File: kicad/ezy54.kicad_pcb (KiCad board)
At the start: 2 copper layers, 141.5 x 124.7 mm, 63 parts

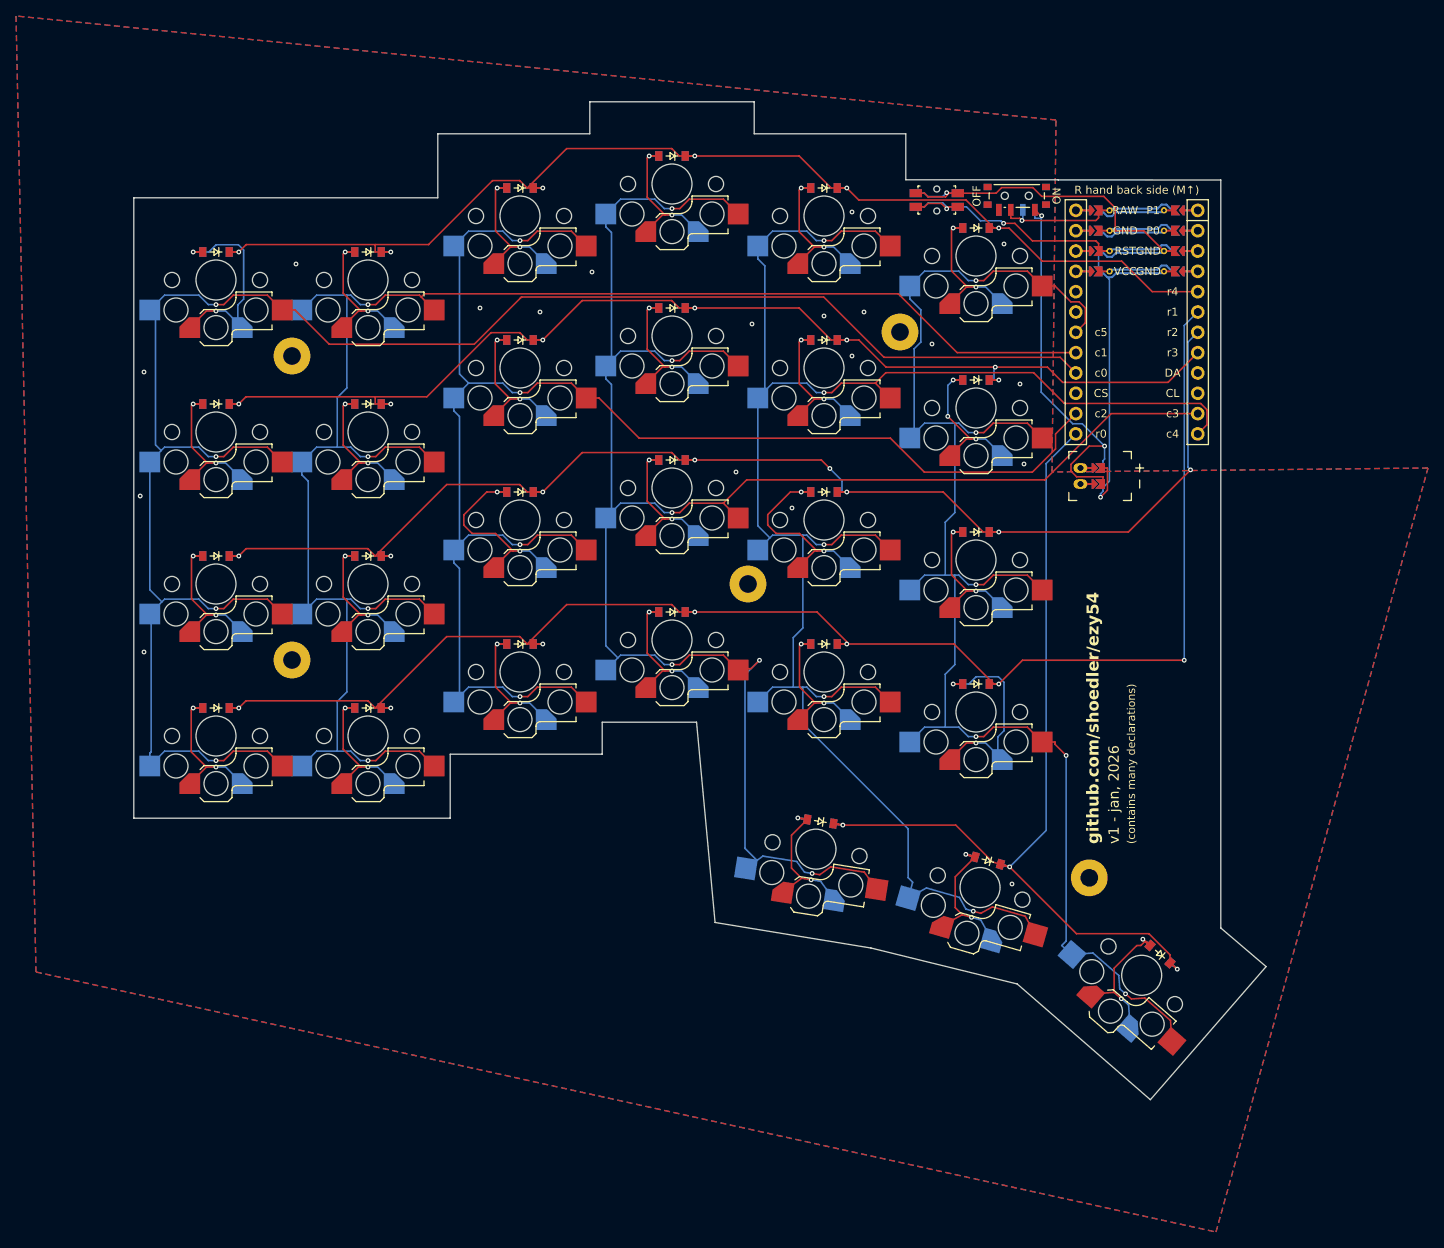
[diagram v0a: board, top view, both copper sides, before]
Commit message: Adds pcb rev1 files
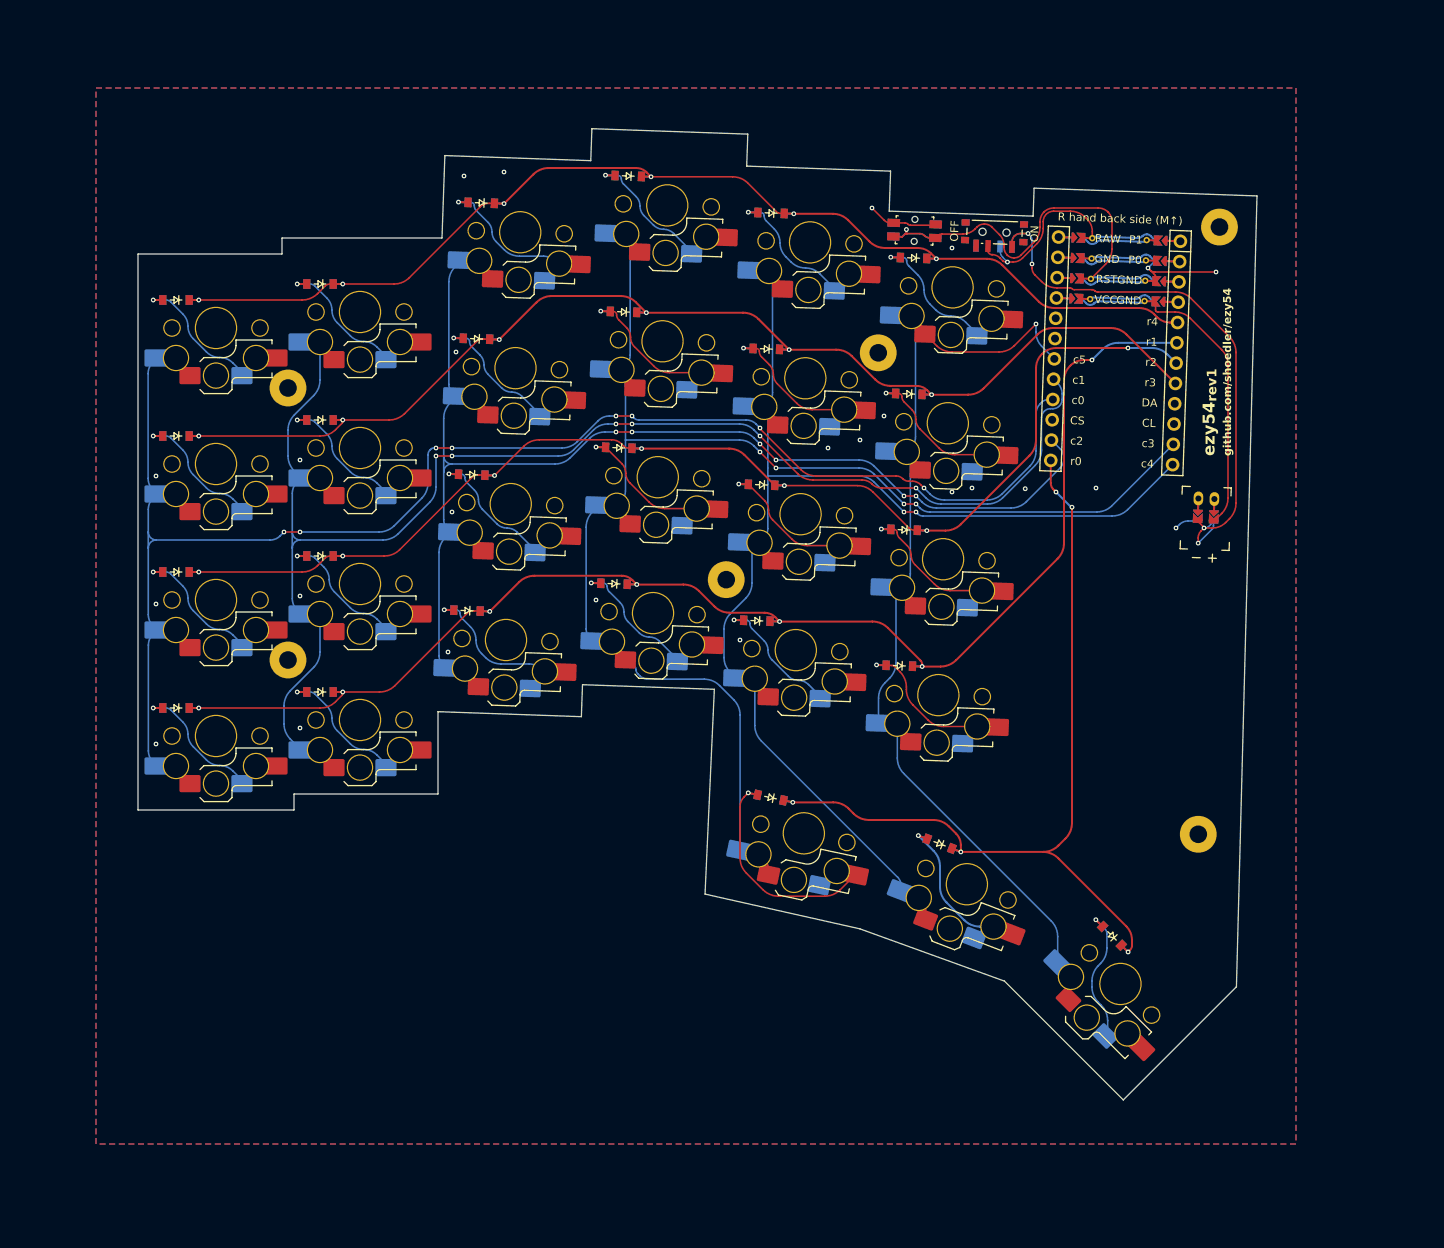
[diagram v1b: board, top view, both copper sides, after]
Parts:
- added MH6: , ceoloide:mounting_hole_npth, F.Cu at (275.4, 86.4)
- moved MH5 64.4 mm to (272.8, 162.3), turned to -2 degrees
- moved MH4 58.7 mm to (213.8, 130.5), turned to -2 degrees
- moved JST1 16.0 mm to (273.8, 120.3), turned to -2 degrees
- moved D21 9.85 mm to (235.4, 141.2), turned to 178 degrees
- moved D22 8.99 mm to (236.0, 124.2), turned to 178 degrees
- moved D17 8.89 mm to (217.6, 135.6), turned to 178 degrees
- moved D24 8.66 mm to (237.2, 90.2), turned to 178 degrees
- moved D23 8.57 mm to (236.6, 107.2), turned to 178 degrees
- moved D13 8.06 mm to (199.8, 131.0), turned to 178 degrees
- moved D18 7.85 mm to (218.2, 118.6), turned to 178 degrees
- moved D9 7.83 mm to (181.4, 134.3), turned to 178 degrees
- moved D4 7.81 mm to (145.0, 95.5)
- moved D20 7.32 mm to (219.4, 84.6), turned to 178 degrees
- moved D19 7.30 mm to (218.8, 101.6), turned to 178 degrees
- moved D8 7.21 mm to (163.0, 93.5)
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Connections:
- S1 pad : (no net) -> GND
- S10 pad : (no net) -> GND
- S11 pad : (no net) -> GND
- S12 pad : (no net) -> GND
- S13 pad : (no net) -> GND
- S14 pad : (no net) -> GND
- S15 pad : (no net) -> GND
- S16 pad : (no net) -> GND
- S17 pad : (no net) -> GND
- S18 pad : (no net) -> GND
- S19 pad : (no net) -> GND
- S2 pad : (no net) -> GND
- S20 pad : (no net) -> GND
- S21 pad : (no net) -> GND
- S22 pad : (no net) -> GND
- S23 pad : (no net) -> GND
- S24 pad : (no net) -> GND
- S25 pad : (no net) -> GND
- S26 pad : (no net) -> GND
- S27 pad : (no net) -> GND
- S3 pad : (no net) -> GND
- S4 pad : (no net) -> GND
- S5 pad : (no net) -> GND
- S6 pad : (no net) -> GND
- S7 pad : (no net) -> GND
- S8 pad : (no net) -> GND
- S9 pad : (no net) -> GND
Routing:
- net c4: track 232.4 -> 169.8 mm, vias 5 -> 2
- net c5: track 193.3 -> 139.5 mm, vias 6 -> 1
- net c3: track 244.2 -> 192.9 mm, vias 6 -> 4
- net c2: track 200.9 -> 165.0 mm, vias 4 -> 6
- net c0: track 239.8 -> 210.5 mm, vias 4 -> 8
- net BAT_P: track 49.8 -> 74.4 mm, vias 2 -> 4
- net GND: track 109.5 -> 86.7 mm, vias 21 -> 25
- net RST: track 42.3 -> 59.9 mm, vias 2 -> 1
- net c1: track 218.8 -> 203.4 mm, vias 4 -> 6
- net c3_r0: track 20.0 -> 33.9 mm, vias 2 -> 1
- net r1: track 188.9 -> 175.8 mm
- net RAW: track 24.7 -> 32.1 mm
- net r3: track 145.9 -> 152.7 mm, vias 7 -> 6
- net r2: track 162.8 -> 157.3 mm, vias 8 -> 7
- net c2_r1: track 19.0 -> 23.3 mm, vias 2 -> 1
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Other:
- board size 141.5 x 124.7 mm -> 139.9 x 121.4 mm
- board text added: "ezy54_{rev1}"
- board text removed: "(contains many declarations)"
- board text removed: "v1 - jan, 2026"
